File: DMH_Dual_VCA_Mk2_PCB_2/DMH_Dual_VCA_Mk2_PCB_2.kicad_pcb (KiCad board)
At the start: 2 copper layers, 48 x 175 mm, 78 parts, among them J1 TS_Jack_6.35mm_Sw, J100 IDC_02x05, J2 TS_Jack_6.35mm_Sw, J200 IDC_02x05, J3 TS_Jack_6.35mm_Sw, J4 TS_Jack_6.35mm_Sw, J5 TS_Jack_6.35mm_Sw, J50 Conn_01x08, J6 TS_Jack_6.35mm_Sw, J60 Conn_01x08, J7 TS_Jack_6.35mm_Sw, J8 TS_Jack_6.35mm_Sw, J9 TS_Jack_6.35mm_Sw, Q1 BC548, Q2 BC548, Q3 BC548, Q4 BC548, U1 TL074, U2 TL074, U3 TL072

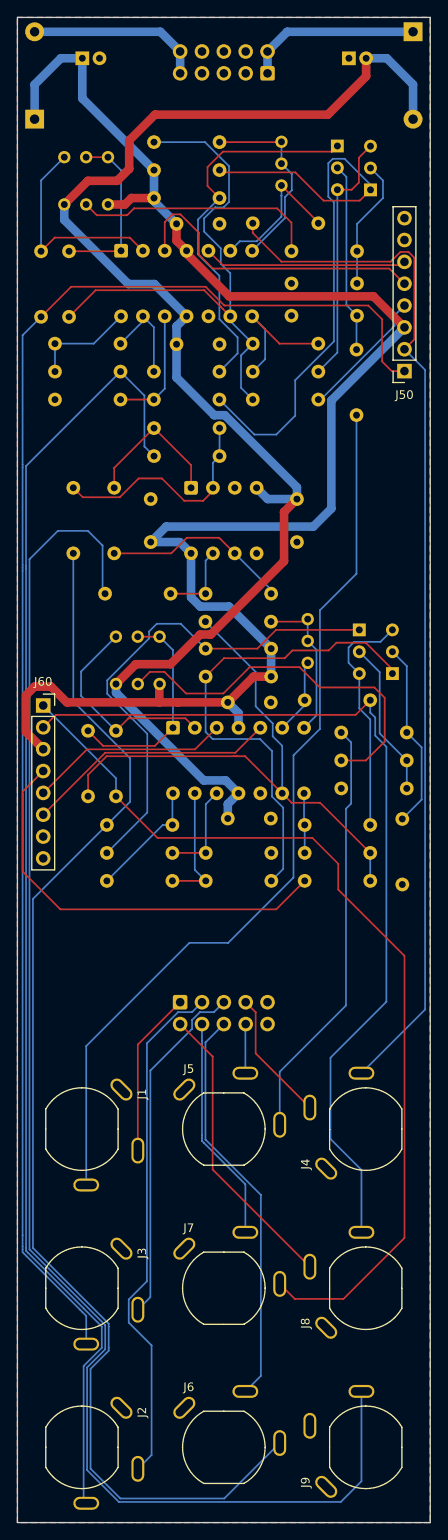
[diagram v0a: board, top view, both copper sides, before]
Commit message: Routed PCB 3
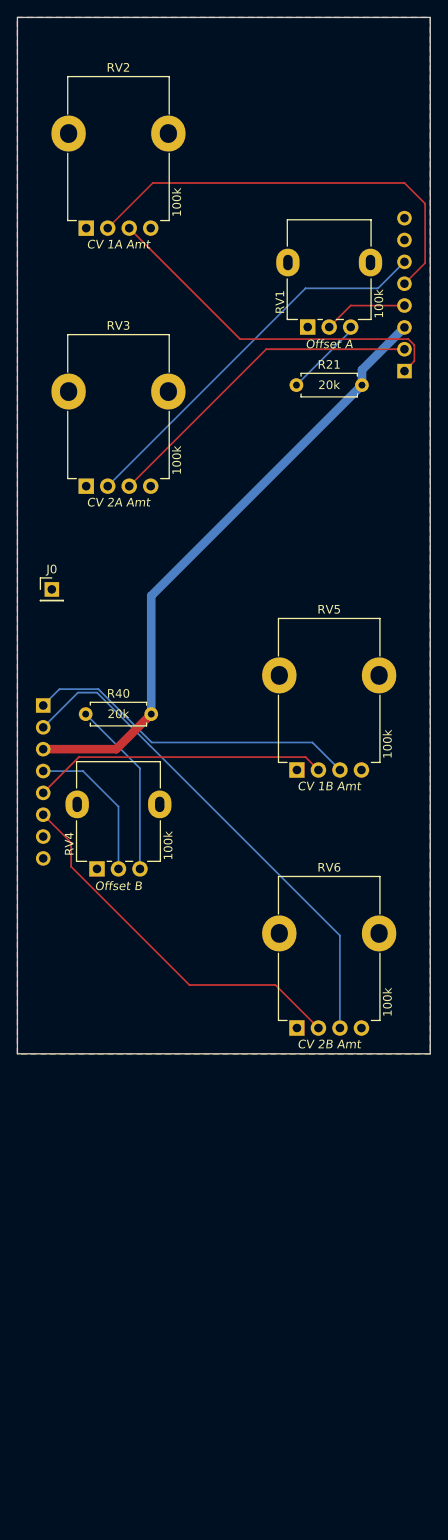
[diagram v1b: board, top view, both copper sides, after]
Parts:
- removed C1, C2: 47uF, Capacitor_THT:CP_Radial_D5.0mm_P2.00mm
- removed C3, C4, C5, C6, C7, C8: 100nF, Capacitor_THT:C_Disc_D4.3mm_W1.9mm_P5.00mm
- removed D1: SB140+, Diode_THT:D_DO-41_SOD81_P10.16mm_Horizontal
- removed D2: SB140-, Diode_THT:D_DO-41_SOD81_P10.16mm_Horizontal
- removed J1, J2, J3, J4, J5, J6, J7, J8, J9: TS_Jack_6.35mm_Sw, SynthStuff:CUI_MJ-63052A
- removed J100: IDC_02x05, SynthStuff:IDC-Header_2x05_P2.54mm_Vertical_Eurorack
- removed J200: IDC_02x05, SynthStuff:IDC-Header_2x05_P2.54mm_Vertical_BackBone
- removed Q1, Q2, Q3, Q4: BC548, Package_TO_SOT_THT:TO-92L_Inline_Wide
- removed R1, R24, R32, R4: 33k, Resistor_THT:R_Axial_DIN0207_L6.3mm_D2.5mm_P7.62mm_Horizontal
- removed R10, R13, R35, R36: 100R, Resistor_THT:R_Axial_DIN0207_L6.3mm_D2.5mm_P7.62mm_Horizontal
- removed R11, R12, R18, R19, R25, R28, R3, R31, R33, R34, R38, R41, R42, R46, R47, R48, R49, R50, R6, R7, R8: 100k, Resistor_THT:R_Axial_DIN0207_L6.3mm_D2.5mm_P7.62mm_Horizontal
- removed R14, R15, R22, R23: 20k, Resistor_THT:R_Axial_DIN0207_L6.3mm_D2.5mm_P7.62mm_Horizontal
- removed R16, R17, R26, R30, R39, R9: 10k, Resistor_THT:R_Axial_DIN0207_L6.3mm_D2.5mm_P7.62mm_Horizontal
- removed R20, R29, R51: 1k, Resistor_THT:R_Axial_DIN0207_L6.3mm_D2.5mm_P7.62mm_Horizontal
- removed RV10, RV11, RV12, RV9: 50k, Potentiometer_THT:Potentiometer_Bourns_3296W_Vertical
- removed RV7, RV8: 100k, Potentiometer_THT:Potentiometer_Bourns_3296W_Vertical
- removed U1, U2: TL074, Package_DIP:DIP-14_W7.62mm_Socket
- removed U3: TL072, Package_DIP:DIP-8_W7.62mm_Socket
- added J0: Conn_01x01, Connector_PinHeader_2.54mm:PinHeader_1x01_P2.54mm_Vertical, F.Cu at (55.0, 109.0)
- added R21: 20k, Resistor_THT:R_Axial_DIN0207_L6.3mm_D2.5mm_P7.62mm_Horizontal, F.Cu at (83.4, 85.2)
- added R40: 20k, Resistor_THT:R_Axial_DIN0207_L6.3mm_D2.5mm_P7.62mm_Horizontal, F.Cu at (58.9, 123.5)
- added RV1: 100k, SynthStuff:Potentiometer_Alpha_RD901F-40-00D_Single_Vertical, F.Cu at (84.8, 78.5)
- added RV2: 100k, SynthStuff:Potentiometer_TT_P110KH1, F.Cu at (60.2, 67.0)
- added RV3: 100k, SynthStuff:Potentiometer_TT_P110KH1, F.Cu at (60.2, 97.0)
- added RV4: 100k, SynthStuff:Potentiometer_Alpha_RD901F-40-00D_Single_Vertical, F.Cu at (60.2, 141.5)
- added RV5: 100k, SynthStuff:Potentiometer_TT_P110KH1, F.Cu at (84.8, 130.0)
- added RV6: 100k, SynthStuff:Potentiometer_TT_P110KH1, F.Cu at (84.8, 160.0)
- J50, J60: footprint Connector_PinSocket_2.54mm:PinSocket_1x08_P2.54mm_Vertical -> Connector_PinHeader_2.54mm:PinHeader_1x08_P2.54mm_Vertical; moved to B.Cu
- turned J50 to 0 degrees
- turned J60 to 180 degrees
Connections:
- J50 pad 1: /Core Circuit A/CV 1 A Input -> /Inputs and Outputs/CV 1 A Jack
- J50 pad 2: /Core Circuit A/CV 2 A Input -> /Inputs and Outputs/CV 2 A Jack
- J50 pad 4: /Core Circuit A/Offset A Pot -> /Inputs and Outputs/Offset A Pot
- J50 pad 5: /Core Circuit A/CV 1 A Pot -> /Inputs and Outputs/CV 1 A Pot
- J50 pad 6: /Core Circuit A/CV 2 A Pot -> /Inputs and Outputs/CV 2 A Pot
- J60 pad 1: /Core Circuit B/CV 1 B Input -> /Inputs and Outputs/CV 1 B Jack
- J60 pad 2: /Core Circuit B/CV 2 B Input -> /Inputs and Outputs/CV 2 B Jack
- J60 pad 4: /Core Circuit B/Offset B Pot -> /Inputs and Outputs/Offset B Pot
- J60 pad 5: /Core Circuit B/CV 1 B Pot -> /Inputs and Outputs/CV 1 B Pot
- J60 pad 6: /Core Circuit B/CV 2 B Pot -> /Inputs and Outputs/CV 2 B Pot
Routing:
- net /Core Circuit A/CV 1 A Input: track 174.0 -> 0.00 mm
- net /Inputs and Outputs/Mix Out Jack: track 171.6 -> 0.00 mm
- net -12V: track 167.1 -> 0.00 mm
- net /Core Circuit A/Output A: track 152.2 -> 0.00 mm
- net /Core Circuit B/Output B: track 144.5 -> 0.00 mm
- net /Core Circuit A/CV 2 A Input: track 121.4 -> 0.00 mm
- net +12V: track 189.3 -> 71.4 mm
- net /Core Circuit B/CV 1 B Input: track 108.0 -> 0.00 mm
- net /Core Circuit B/CV 2 B Input: track 106.1 -> 0.00 mm
- net /Core Circuit A/Input A: track 105.2 -> 0.00 mm
- net Net-(Q2-C): track 69.4 -> 0.00 mm
- net Net-(U2C--): track 67.8 -> 0.00 mm
- net Net-(U1C--): track 63.6 -> 0.00 mm
- net Net-(J200-Pin_2): track 60.5 -> 0.00 mm
- net /Inputs and Outputs/CV 2 B Jack: track 0.00 -> 58.6 mm
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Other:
- board size 48 x 175 mm -> 48 x 120.5 mm
